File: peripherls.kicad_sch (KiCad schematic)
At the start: 21 parts, among them J6 NS6312, Q1 2N7002H, Q3 BD237, SW1 SW_MEC_5E, SW3 SW_MEC_5E, U2 STM32G070KBTx

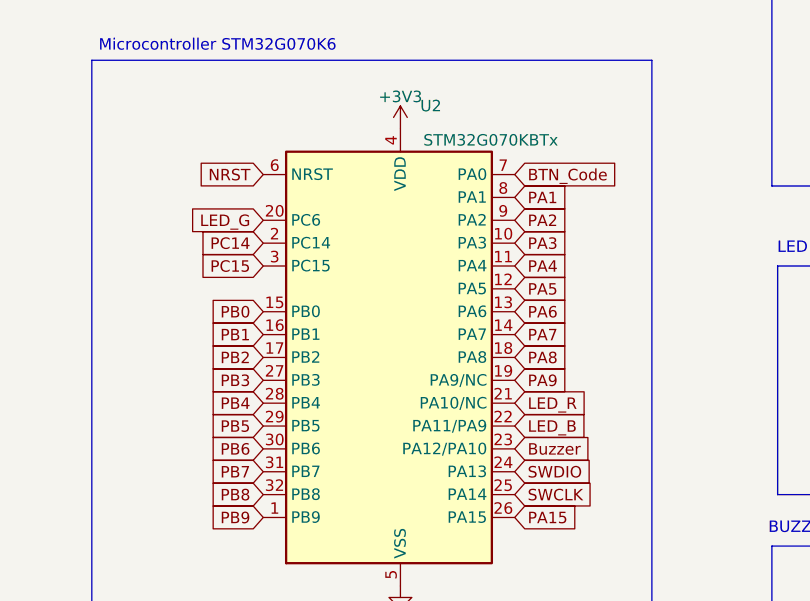
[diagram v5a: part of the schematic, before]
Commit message: board v1
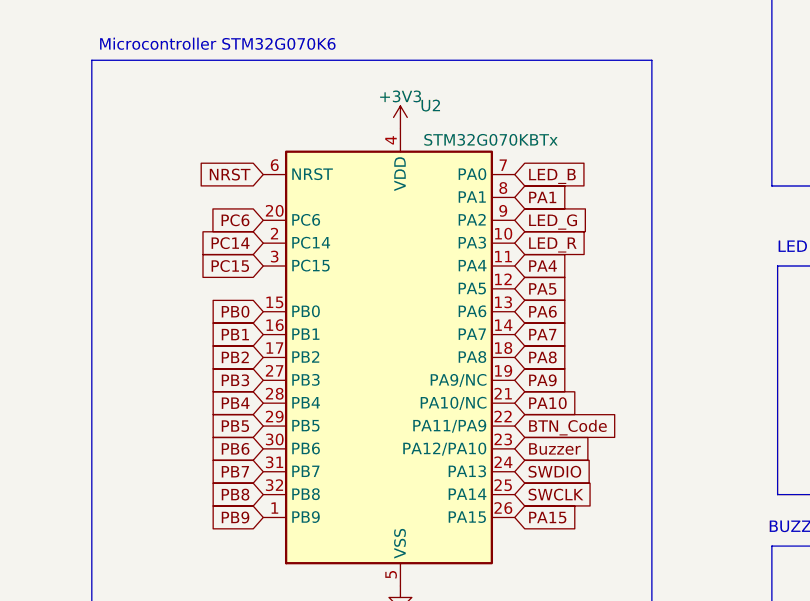
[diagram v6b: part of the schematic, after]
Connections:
- net PA2 is gone; now on net LED_G: U2.9 (PA2)
- net PA3 is gone; now on net LED_R: U2.10 (PA3)
- net BTN_Code: now also U2.22 (PA11/PA9); no longer U2.7 (PA0)
- net LED_B: now also U2.7 (PA0); no longer U2.22 (PA11/PA9)
- net LED_G: no longer U2.20 (PC6)
- net LED_R: no longer U2.21 (PA10/NC)
- new net PA10: U2.21 (PA10/NC)
- new net PC6: U2.20 (PC6)
